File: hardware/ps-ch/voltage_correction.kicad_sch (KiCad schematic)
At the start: 35 parts, among them Q10 MMBT3904, Q5 MMBT3906, Q6 MMBT3906, Q7 MMBT3904, Q8 MMBT3904, U7 OPA992IDCKR, U8 OPA992IDCKR

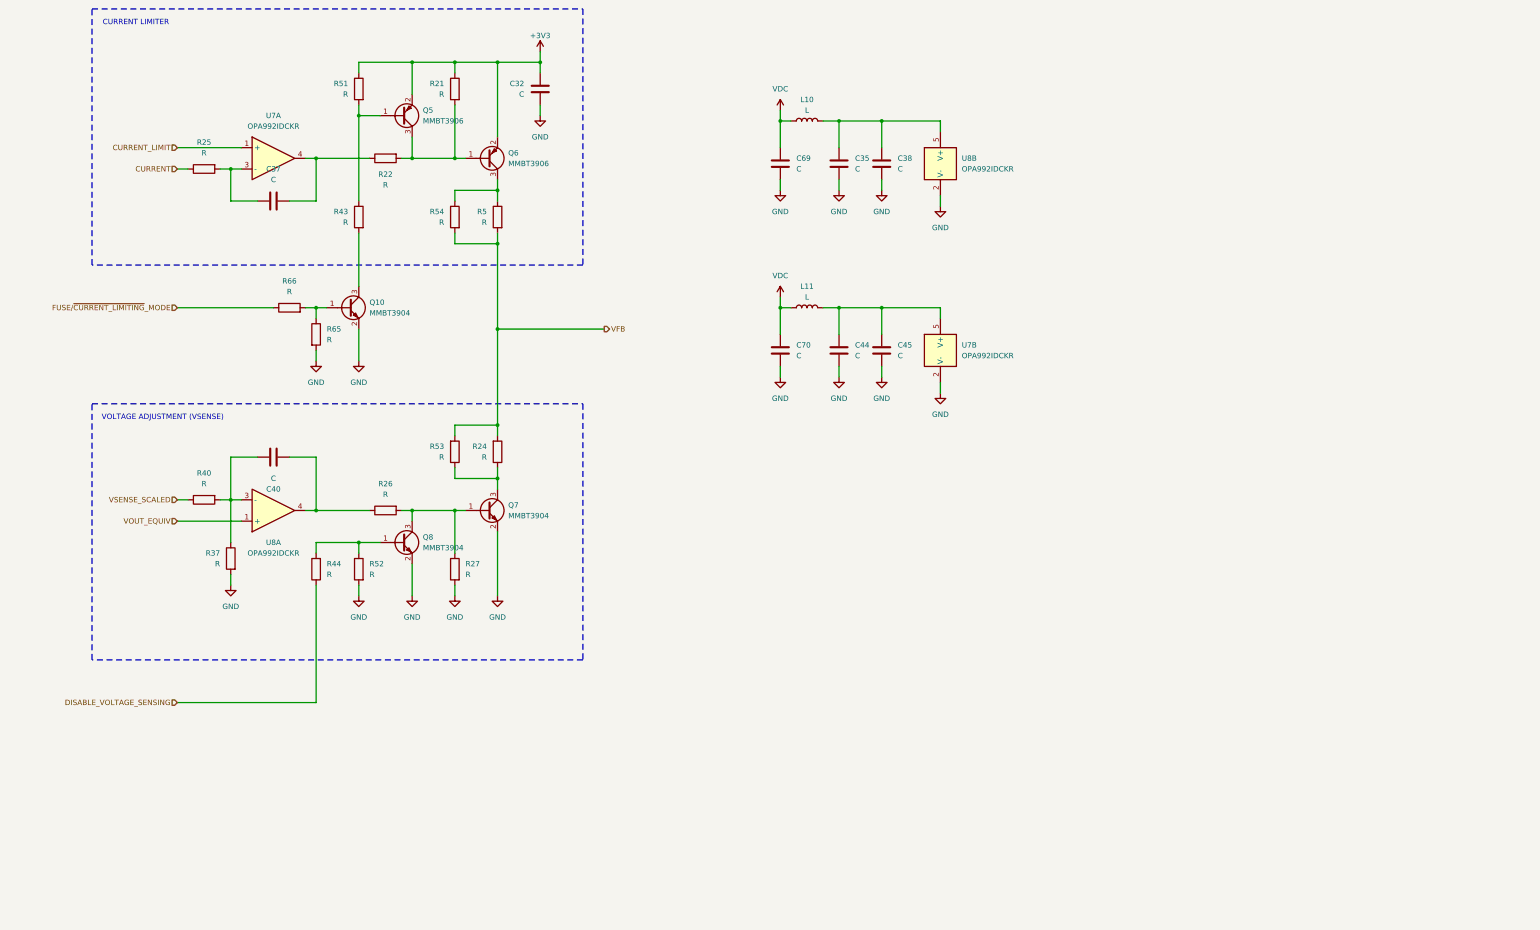
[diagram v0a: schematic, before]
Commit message: did some wiring
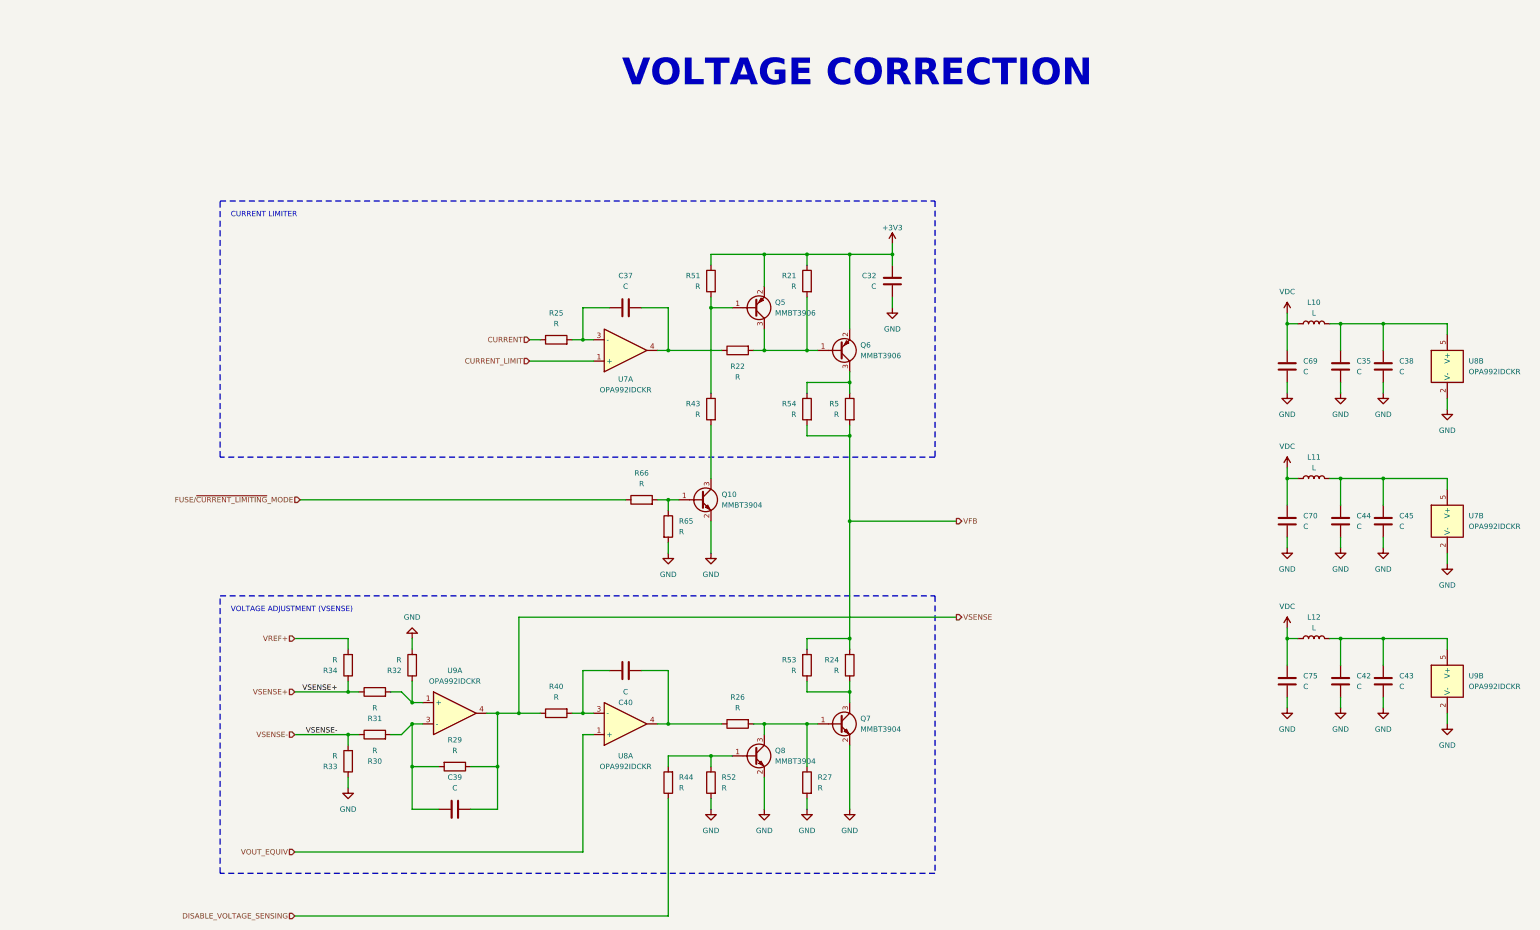
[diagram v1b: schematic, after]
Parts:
- removed R37: R, symbol Device:R
- added C39, C42, C43, C75: C, symbol Device:C
- added L12: L, symbol Device:L
- added R29, R30, R31, R32, R33, R34: R, symbol Device:R
- added U9: OPA992IDCKR, symbol ps-ch:OPA992IDCKR
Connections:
- net GND: now also C42.2, C43.2, C75.2, R32.2, R33.1, U9.2 (V-)
- net VDC: now also C75.1, L12.1
- net VSENSE_SCALED renamed VSENSE
- net VSENSE: now also C39.1, R29.1, U9.4
- new net: R31.2, R32.1, U9.1 (+)
- new net: C39.2, R29.2, R30.2, U9.3 (-)
- new net: C42.1, C43.1, L12.2, U9.5 (V+)
- new net VREF+: R34.2
- new net VSENSE+: R31.1, R34.1
- new net VSENSE-: R30.1, R33.2
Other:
- note added: "VOLTAGE CORRECTION"
- moved on the sheet: C32, C35, C37, C38, C40, C44, C45, C69, C70, L10, L11, Q10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
